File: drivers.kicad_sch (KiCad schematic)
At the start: 14 parts, among them J7 Conn_Coaxial, J8 Conn_Coaxial, U6 LM358

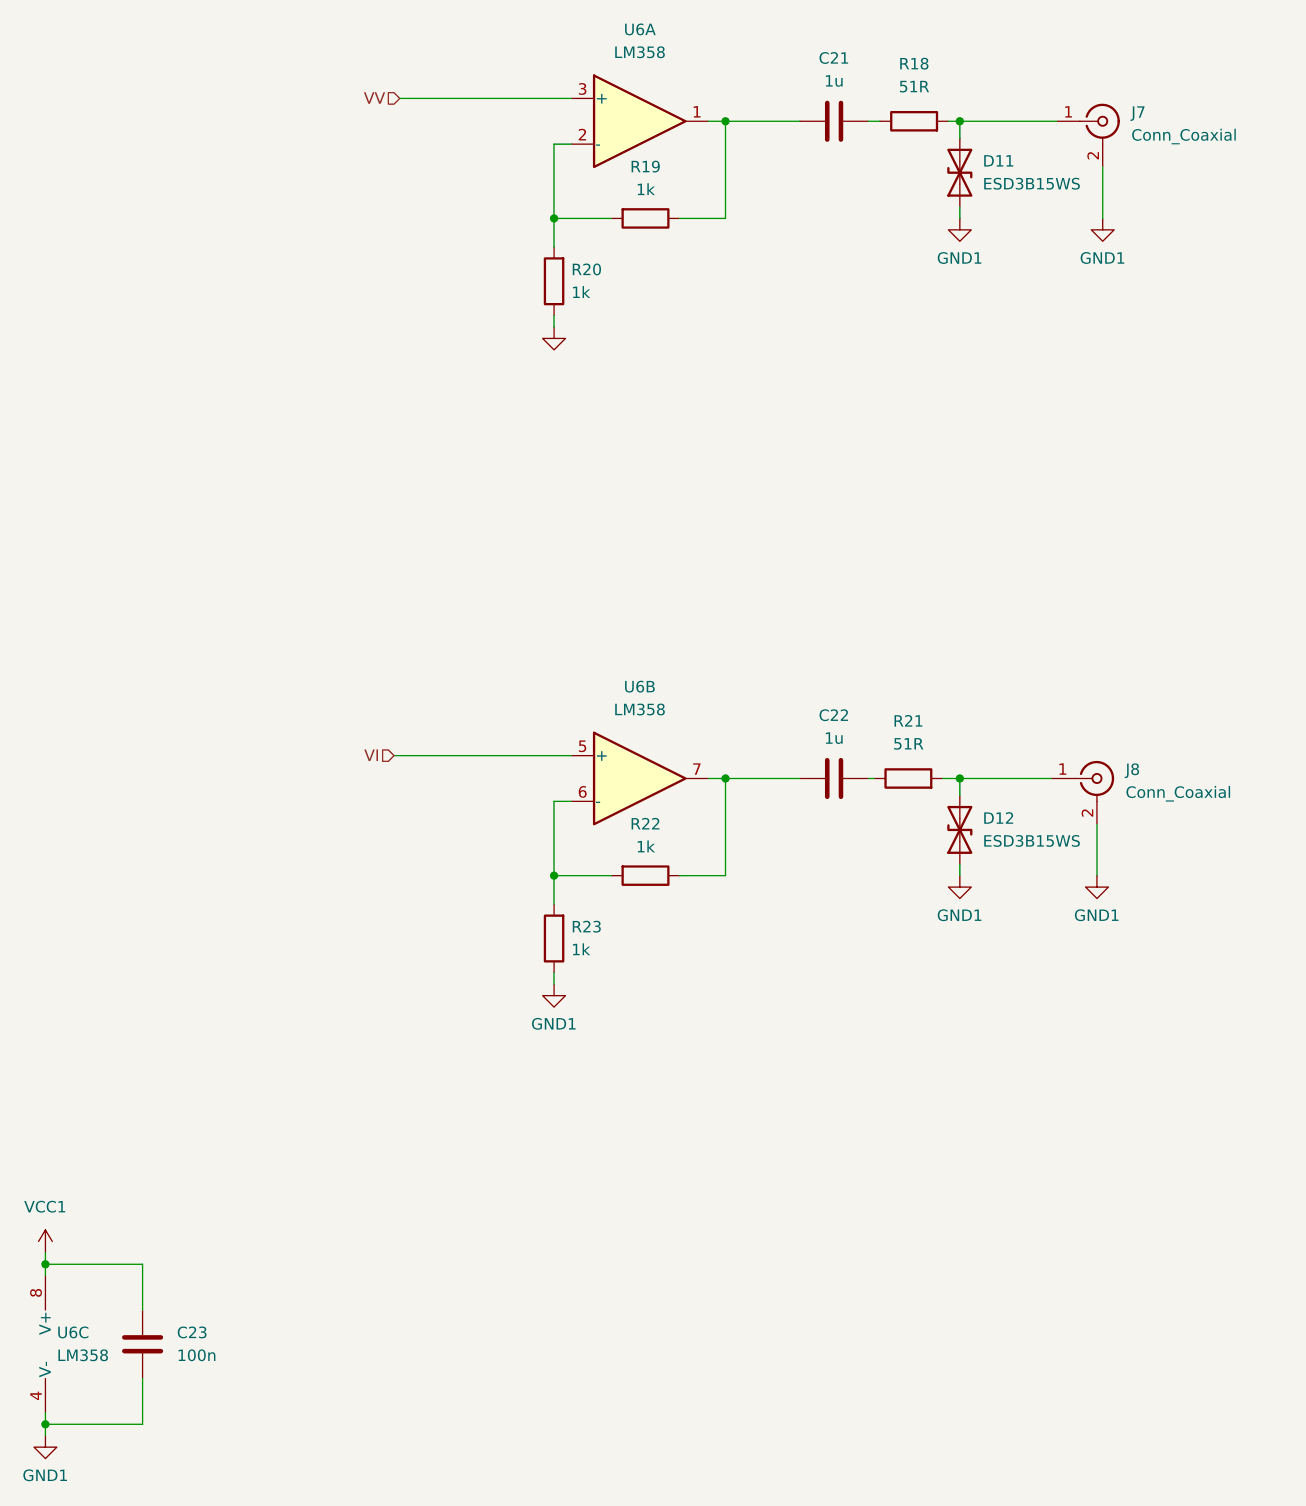
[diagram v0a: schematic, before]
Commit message: Redesign pcb
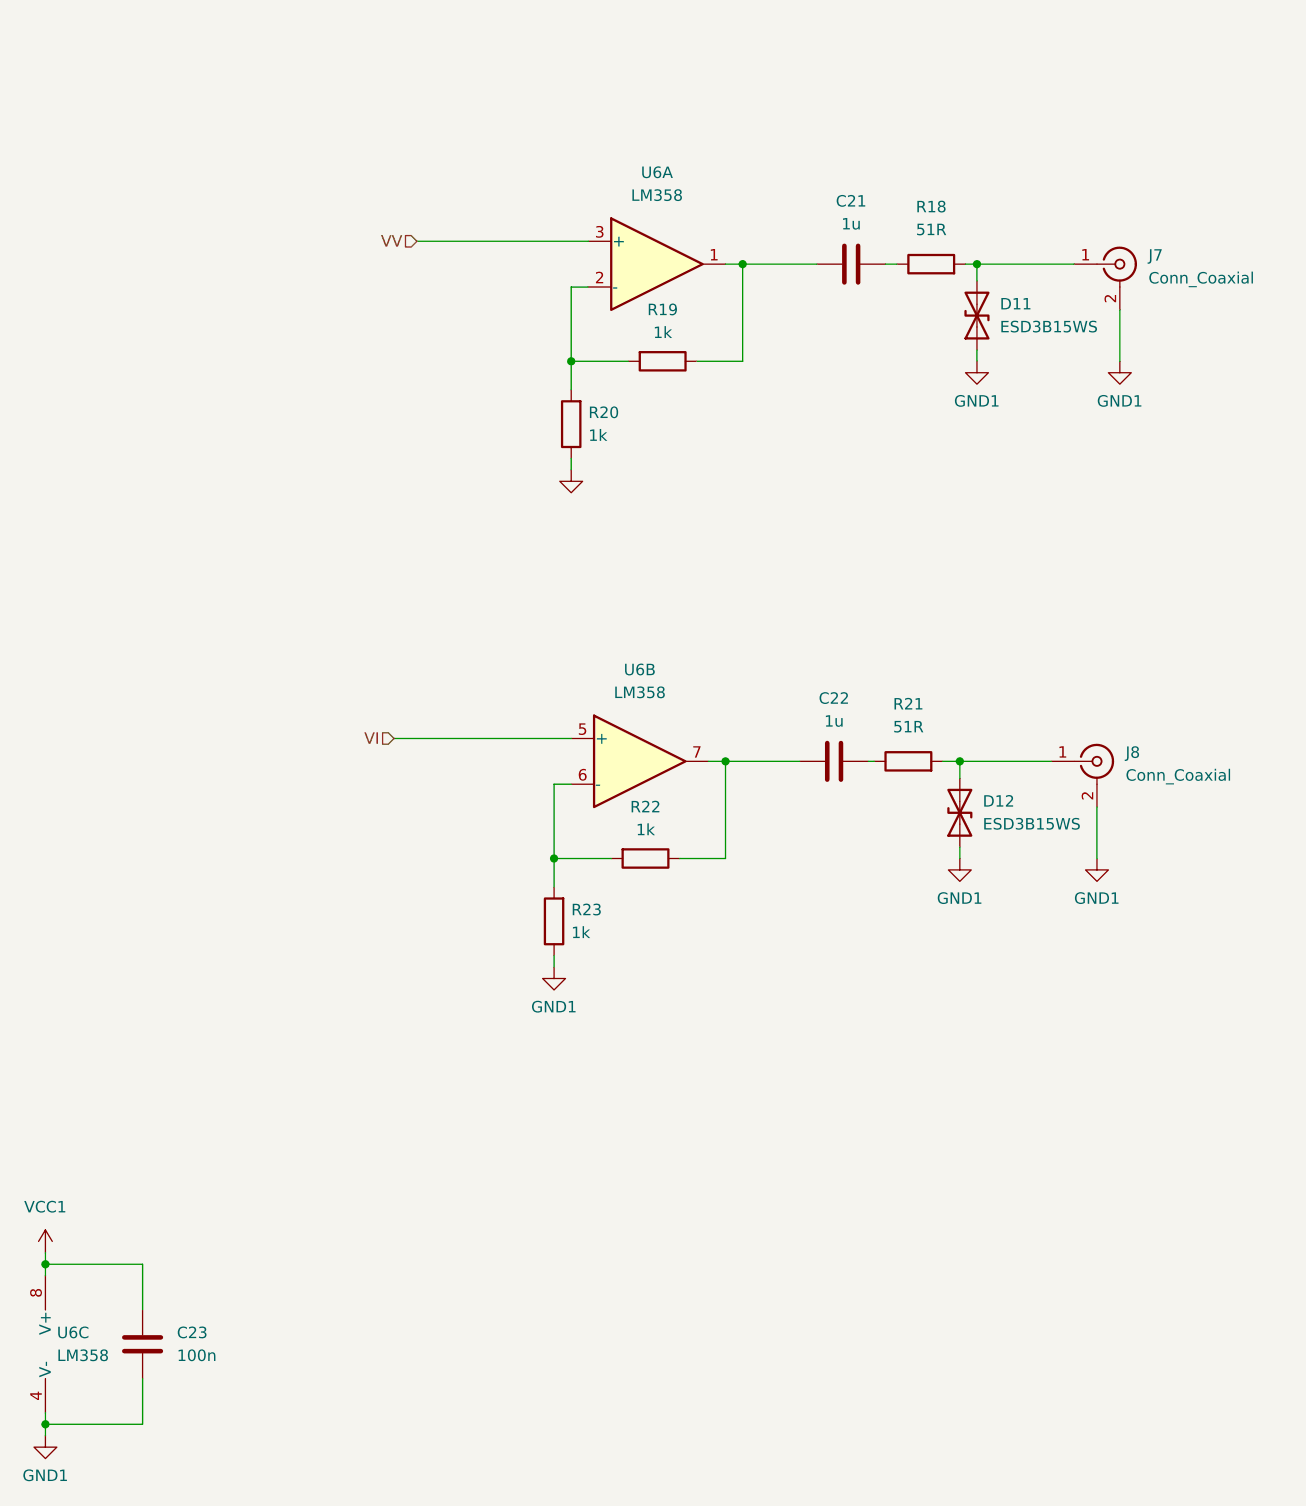
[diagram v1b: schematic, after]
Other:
- moved on the sheet: C21, C22, D11, D12, J7, J8, R18, R19, R20, R21, R22, R23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

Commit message: Bump revision to 1.1.0
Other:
- company: (none) -> koszalix
- title: (none) -> lineScope Isolators 
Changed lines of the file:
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@@
 	(generator_version "8.0")
 	(paper "A4")
+	(title_block
+		(title "lineScope Isolators ")
+		(date "2024-05-26")
+		(rev "Rev 1.1.0")
+		(company "koszalix")
+	)
 	(junction
 		(at 121.285 107.315)
